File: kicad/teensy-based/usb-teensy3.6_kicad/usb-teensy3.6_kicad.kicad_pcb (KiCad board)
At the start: 2 copper layers, 154.9 x 90.2 mm, 24 parts, among them SW1 SW_Push, SW2 SW_Push, U1 Teensy3.6

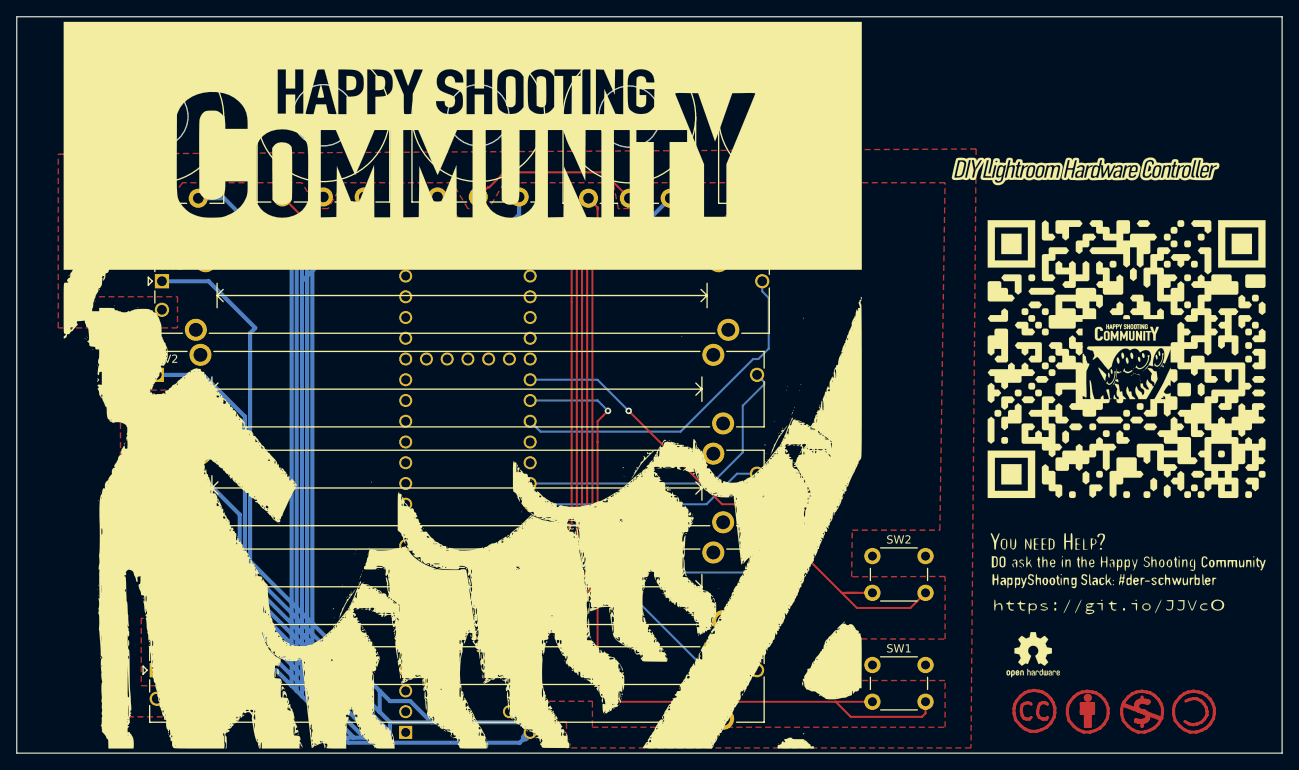
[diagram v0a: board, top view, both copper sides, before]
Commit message: mod render without parts
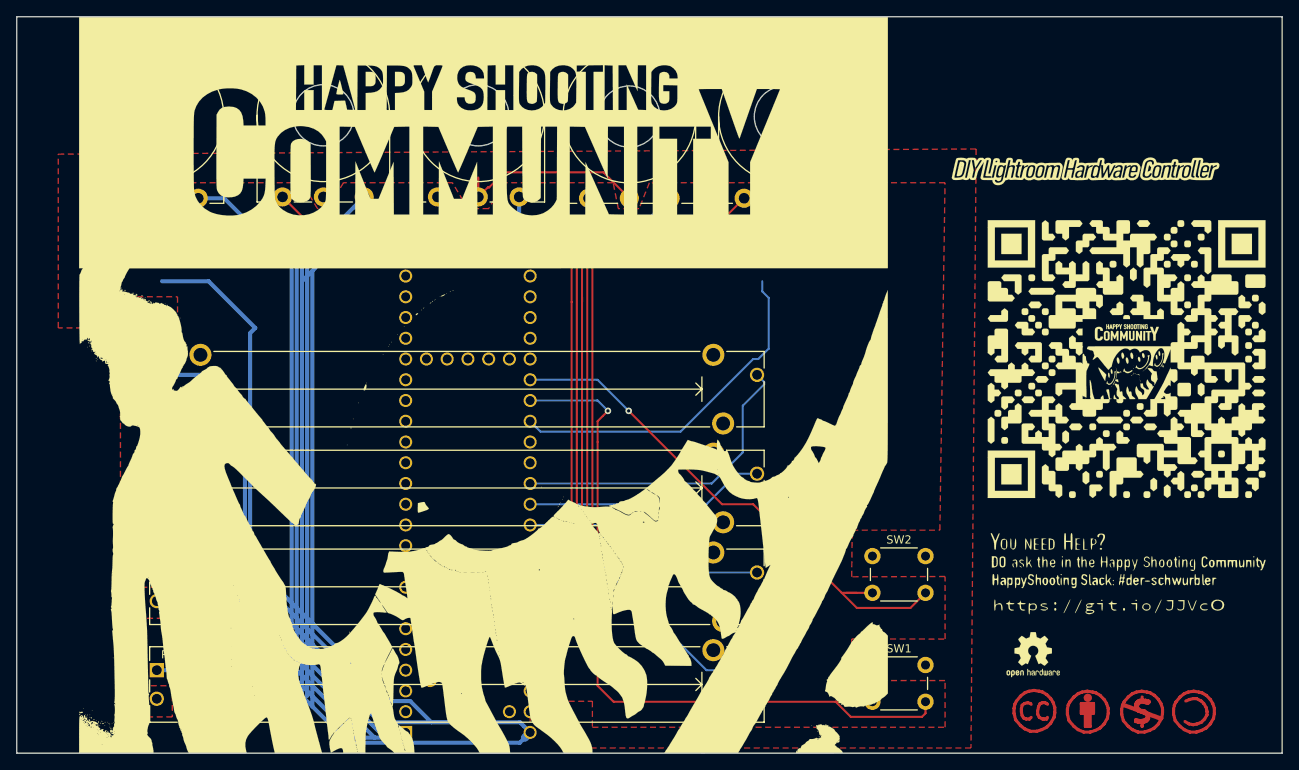
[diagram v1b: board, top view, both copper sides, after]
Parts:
- removed the G*** at (128.3, 104.8)
- removed the G*** at (127.6, 104.8)
- removed RV1: 10k sl, Potentiometer_THT:Potentiometer_Bourns_PTA6043_Single_Slide
- added G***: LOGO, HappyShooting:hsc_diff_print_i_375, F.Cu at (130.8, 104.8)
- added G***: LOGO, HappyShooting:hsc_silk_375, F.Cu at (130.8, 104.8)
